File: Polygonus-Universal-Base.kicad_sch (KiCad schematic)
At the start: 11 parts, among them J1 Conn_02x04_Top_Bottom, J4 Polygonus_Plugs, J5 Conn_02x04_Top_Bottom, U1 WBO-Single-Module, U14 WBO-Single-Module

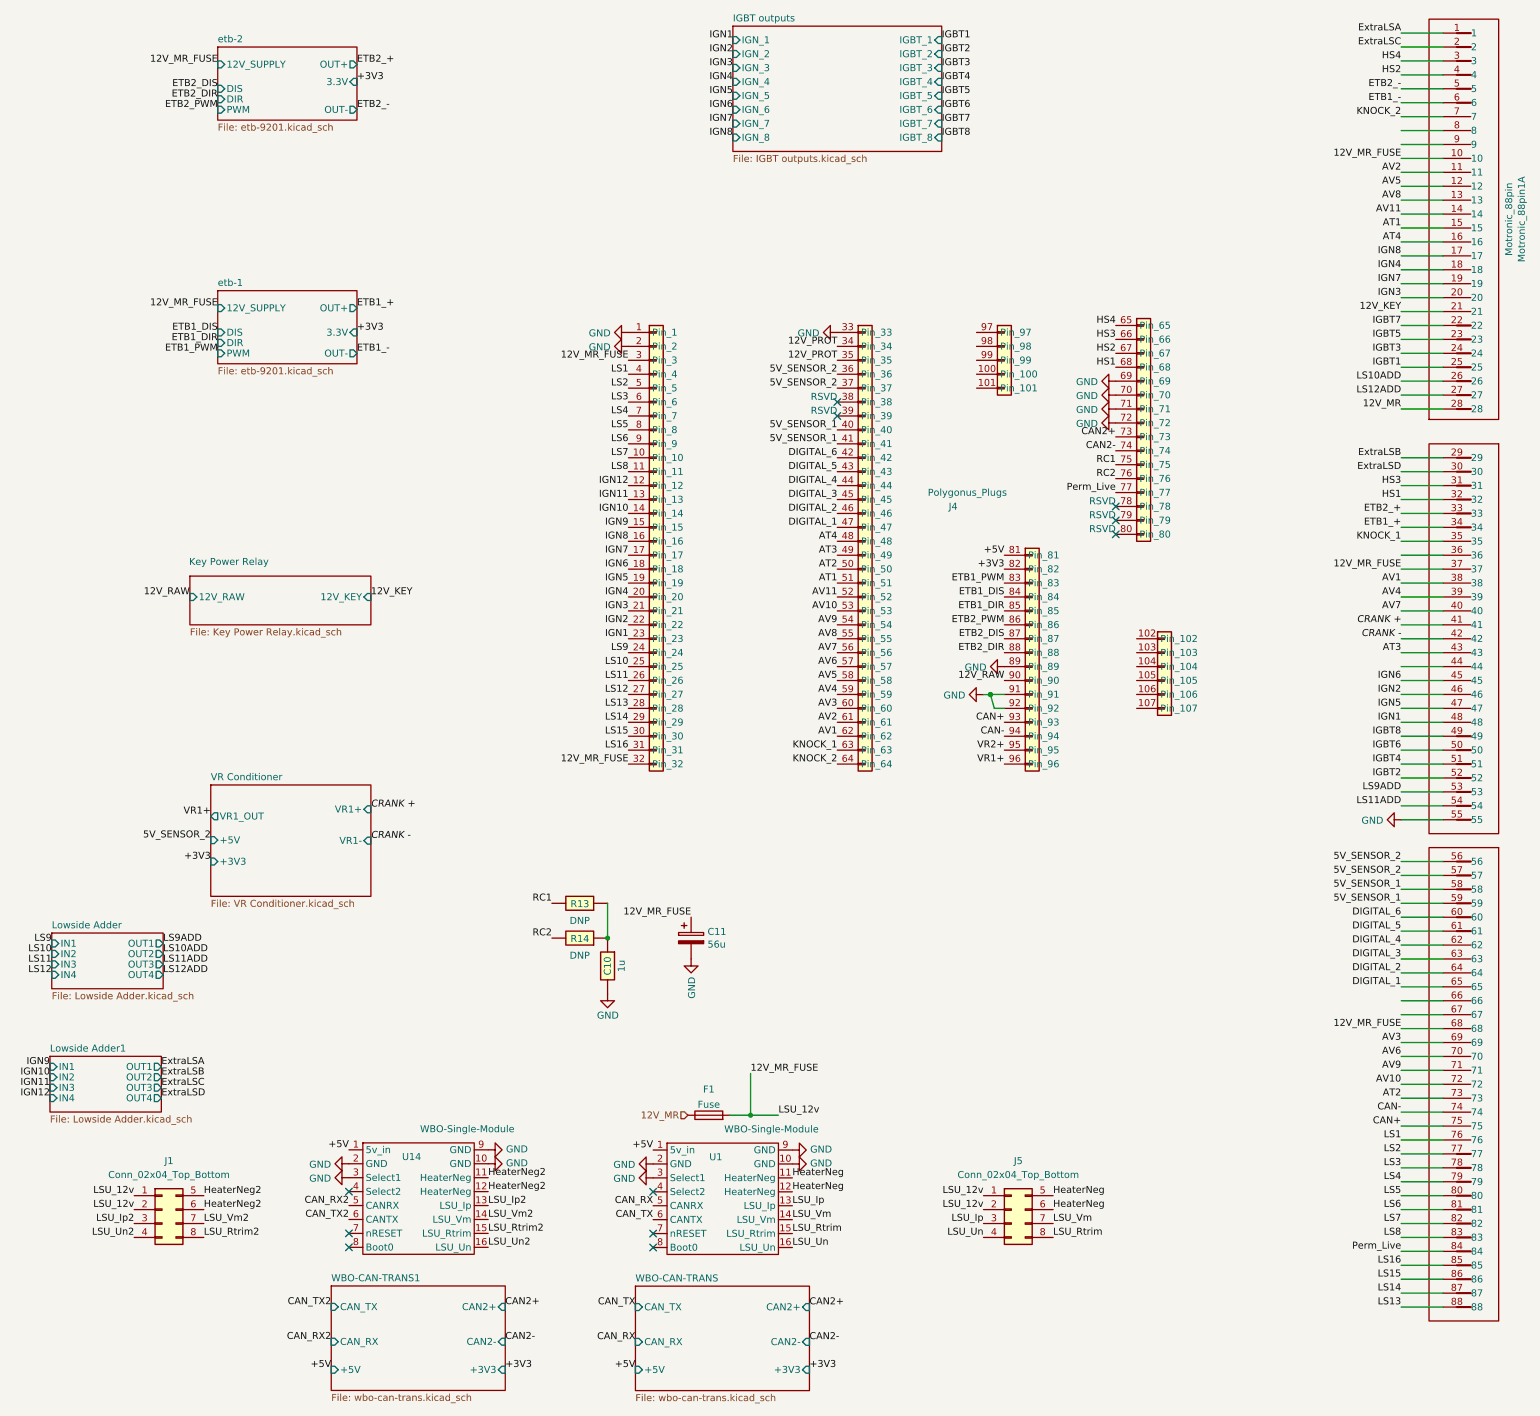
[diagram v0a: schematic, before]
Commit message: updated and fixed, check JLC exports
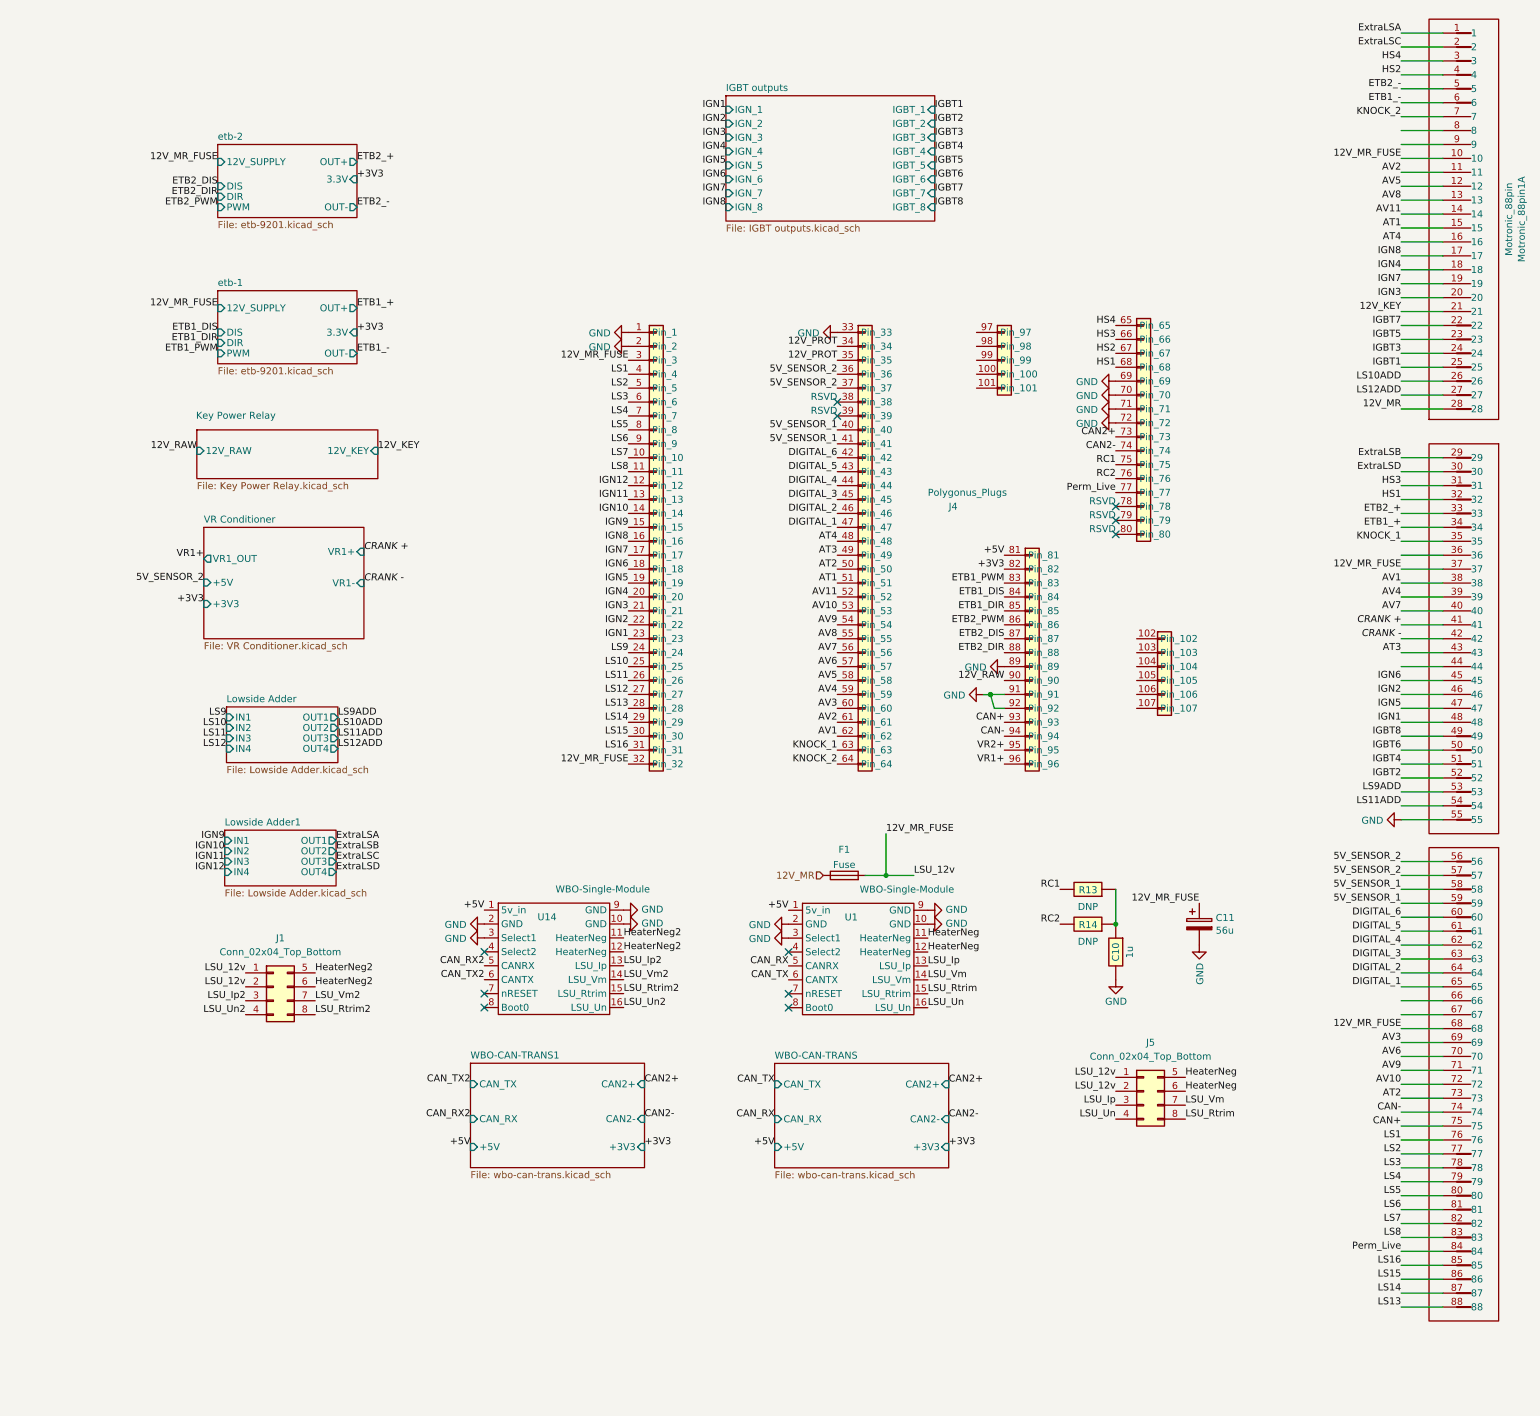
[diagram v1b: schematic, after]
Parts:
- J4: footprint Simon:Polygonus_Plugs -> Simon:Polygonus-With-USB-SWD
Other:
- moved on the sheet: C10, C11, F1, J1, J5, R13, R14, U1, U14

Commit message: All fixed up for JLC
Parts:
- C10, R13, R14: LCSC C23241 -> DNP
- F1: LCSC (none) -> C5249699
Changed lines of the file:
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@@
       (effects (font (size 1.27 1.27)) hide)
     )
-    (property "LCSC" "C23241" (id 4) (at 219.71 186.69 0)
+    (property "LCSC" "DNP" (id 4) (at 219.71 186.69 0)
       (effects (font (size 1.27 1.27)) hide)
     )
@@
       (effects (font (size 1.27 1.27)) hide)
     )
-    (property "LCSC" "C23241" (id 4) (at 219.71 193.04 0)
+    (property "LCSC" "DNP" (id 4) (at 219.71 193.04 0)
       (effects (font (size 1.27 1.27)) hide)
     )
@@
       (effects (font (size 1.27 1.27)) hide)
     )
+    (property "LCSC" "C5249699" (id 4) (at 170.18 184.15 90)
+      (effects (font (size 1.27 1.27)) hide)
+    )
     (pin "1")
     (pin "2")
@@
       (effects (font (size 1.27 1.27)) hide)
     )
-    (property "LCSC" "C23241" (id 4) (at 219.71 193.04 0)
-      (effects (font (size 1.27 1.27)) hide)
-    )
+    (property "LCSC" "DNP" (id 4) (at 219.71 193.04 0)
+      (effects (font (size 1.27 1.27)) hide)
+    )
